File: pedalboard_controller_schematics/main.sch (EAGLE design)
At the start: 53 parts, among them IC1 74LS139N, IC2 74LS148N, IC3 7805TV, IC4 74LS279N, K1 TQ2-L-5V, K2 TQ2-L-5V, K3 TQ2-L-5V, K4 TQ2-L-5V, SW0 SWITCH-SPST, SW1 SWITCH-SPST, SW2 SWITCH-SPST, SW3 SWITCH-SPST, SW4 SWITCH-SPST, SW5 SWITCH-SPST, SW6 SWITCH-SPST, SW7 SWITCH-SPST, U1 LPC1114FN28/102, U2 UA78MC

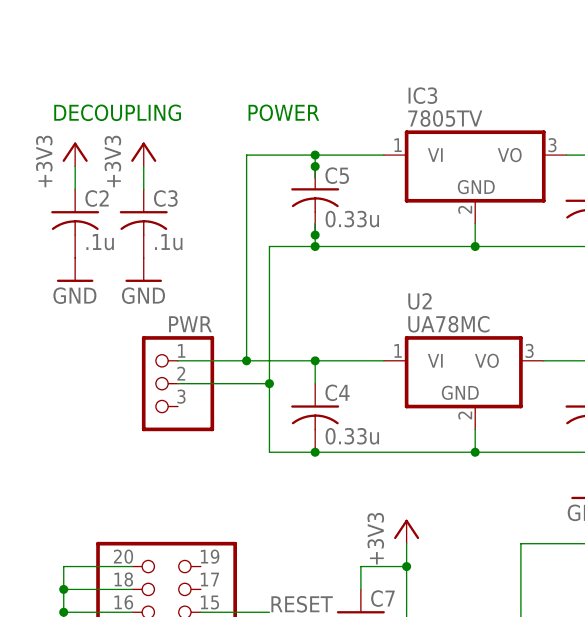
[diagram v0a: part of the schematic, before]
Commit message: updated main board
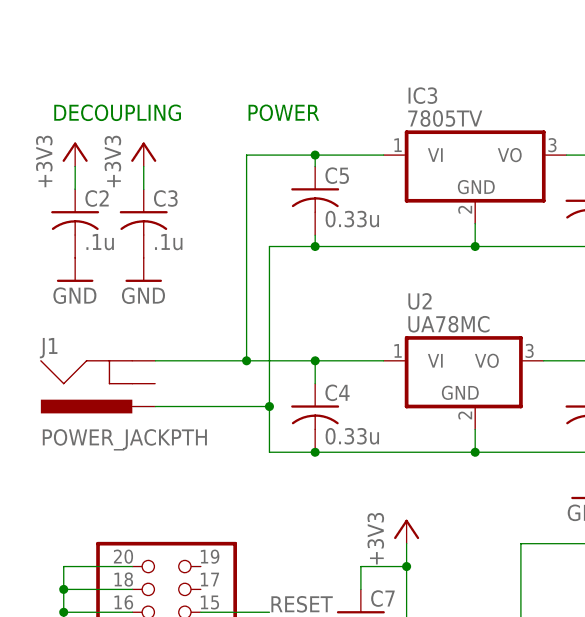
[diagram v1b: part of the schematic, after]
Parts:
- removed PWR: (no value), pinhead:PINHD-1X3
- added J1: POWER_JACKPTH, SparkFun-Connectors:POWER_JACKPTH
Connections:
- net GND: now also J1.PWR; no longer PWR.2
- net N$2: now also J1.GND; no longer PWR.1
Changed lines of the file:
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@@
 <part name="IC2" library="74xx-us" deviceset="74*148" device="N" technology="LS"/>
 <part name="U1" library="lpc_11xx" deviceset="LPC1114FN28/102" device=""/>
-<part name="PWR" library="pinhead" deviceset="PINHD-1X3" device=""/>
 <part name="U2" library="lpc_11xx" deviceset="UA78M*C" device=""/>
 <part name="C1" library="rcl" deviceset="C-US" device="050-024X044" value="0.1u"/>
@@
 <part name="R14" library="resistor" deviceset="R-US_" device="0204/7" value="4.7K"/>
 <part name="R15" library="resistor" deviceset="R-US_" device="0204/7" value="4.7K"/>
+<part name="J1" library="SparkFun-Connectors" deviceset="POWER_JACK" device="PTH"/>
 </parts>
 <sheets>
@@
 <instance part="IC2" gate="A" x="25.4" y="-17.78"/>
 <instance part="U1" gate="G$1" x="76.2" y="20.32"/>
-<instance part="PWR" gate="A" x="-20.32" y="50.8" rot="MR0"/>
 <instance part="U2" gate="G$1" x="15.24" y="50.8"/>
 <instance part="C1" gate="G$1" x="27.94" y="48.26"/>
@@
 <instance part="R14" gate="G$1" x="0" y="-45.72" rot="MR90"/>
 <instance part="R15" gate="G$1" x="-7.62" y="-45.72" rot="MR90"/>
+<instance part="J1" gate="G$1" x="-22.86" y="55.88" rot="MR180"/>
 </instances>
 <busses>
@@
 <segment>
 <pinref part="U2" gate="G$1" pin="VI"/>
-<pinref part="PWR" gate="A" pin="1"/>
 <pinref part="C4" gate="G$1" pin="1"/>
 <wire x1="5.08" y1="53.34" x2="-2.54" y2="53.34" width="0.1524" layer="91"/>
 <wire x1="-2.54" y1="53.34" x2="-10.16" y2="53.34" width="0.1524" layer="91"/>
-<wire x1="-10.16" y1="53.34" x2="-17.78" y2="53.34" width="0.1524" layer="91"/>
+<wire x1="-10.16" y1="53.34" x2="-20.32" y2="53.34" width="0.1524" layer="91"/>
 <wire x1="-2.54" y1="50.8" x2="-2.54" y2="53.34" width="0.1524" layer="91"/>
 <junction x="-2.54" y="53.34"/>
@@
 <wire x1="-2.54" y1="76.2" x2="-2.54" y2="74.93" width="0.1524" layer="91"/>
 <pinref part="IC3" gate="A1" pin="VI"/>
-<wire x1="-2.54" y1="74.93" x2="-2.54" y2="73.66" width="0.1524" layer="91"/>
 <wire x1="-2.54" y1="76.2" x2="5.08" y2="76.2" width="0.1524" layer="91"/>
 <junction x="-2.54" y="76.2"/>
 <pinref part="C5" gate="G$1" pin="1"/>
-<junction x="-2.54" y="74.93"/>
+<pinref part="J1" gate="G$1" pin="GND"/>
 </segment>
 </net>
@@
 <net name="GND" class="0">
 <segment>
-<wire x1="-17.78" y1="50.8" x2="-7.62" y2="50.8" width="0.1524" layer="91"/>
-<wire x1="-7.62" y1="50.8" x2="-7.62" y2="43.18" width="0.1524" layer="91"/>
+<wire x1="-20.32" y1="48.26" x2="-7.62" y2="48.26" width="0.1524" layer="91"/>
+<wire x1="-7.62" y1="48.26" x2="-7.62" y2="43.18" width="0.1524" layer="91"/>
 <wire x1="-7.62" y1="43.18" x2="-2.54" y2="43.18" width="0.1524" layer="91"/>
 <wire x1="-2.54" y1="43.18" x2="15.24" y2="43.18" width="0.1524" layer="91"/>
@@
 <junction x="27.94" y="43.18"/>
 <pinref part="U2" gate="G$1" pin="GND"/>
-<pinref part="PWR" gate="A" pin="2"/>
 <pinref part="C1" gate="G$1" pin="2"/>
 <pinref part="GND1" gate="1" pin="GND"/>
@@
 <wire x1="15.24" y1="66.04" x2="-2.54" y2="66.04" width="0.1524" layer="91"/>
 <wire x1="-2.54" y1="66.04" x2="-7.62" y2="66.04" width="0.1524" layer="91"/>
-<wire x1="-7.62" y1="66.04" x2="-7.62" y2="50.8" width="0.1524" layer="91"/>
-<junction x="-7.62" y="50.8"/>
-<wire x1="-2.54" y1="68.58" x2="-2.54" y2="67.31" width="0.1524" layer="91"/>
+<wire x1="-7.62" y1="66.04" x2="-7.62" y2="48.26" width="0.1524" layer="91"/>
+<junction x="-7.62" y="48.26"/>
 <junction x="-2.54" y="66.04"/>
 <pinref part="IC3" gate="A1" pin="GND"/>
@@
 <junction x="15.24" y="66.04"/>
 <pinref part="C5" gate="G$1" pin="2"/>
-<junction x="-2.54" y="67.31"/>
-</segment>
-<segment>
+<pinref part="J1" gate="G$1" pin="PWR"/>
+</segment>
+<segment>
